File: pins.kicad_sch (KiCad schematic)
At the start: 21 parts, among them J2 Conn_01x40_Pin, J3 Conn_01x09, Q1 BC817, U11 TXS0108EPW, U8 TXS0102DCU

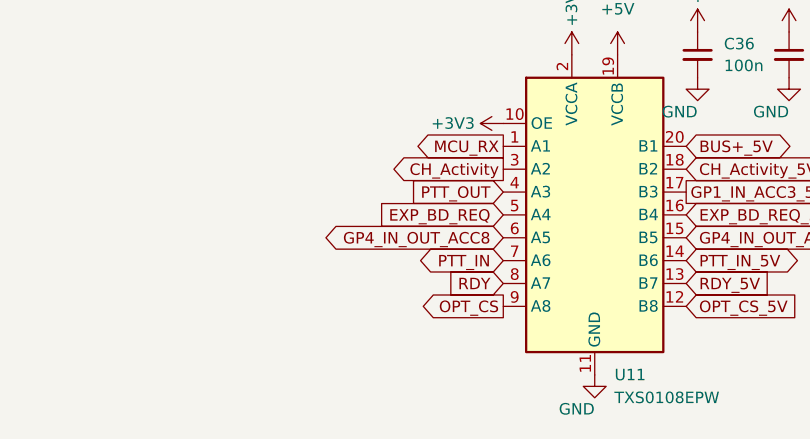
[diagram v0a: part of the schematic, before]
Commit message: end of day commit
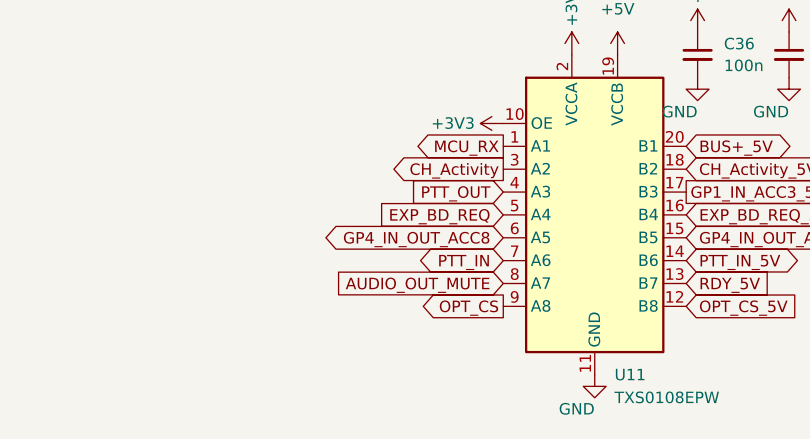
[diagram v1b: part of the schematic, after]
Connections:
- net RDY is gone; now on net AUDIO_OUT_MUTE: U11.8 (A7)
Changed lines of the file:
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@@
+		)
+	)
+	(global_label "AUDIO_OUT_MUTE"
+		(shape input)
+		(at 100.33 171.45 180)
+		(fields_autoplaced yes)
+		(effects
+			(font
+				(size 1.27 1.27)
+			)
+			(justify right)
+		)
+		(property "Intersheetrefs" "${INTERSHEET_REFS}"
+			(at 81.2581 171.45 0)
+			(effects
+				(font
+					(size 1.27 1.27)
+				)
+				(justify right)
+				(hide yes)
+			)
 		)
 	)
@@
 			(effects
 				(font
-					(size 1.27 1.27)
-				)
-				(justify right)
-				(hide yes)
-			)
-		)
-	)
-	(global_label "RDY"
-		(shape input)
-		(at 100.33 171.45 180)
-		(fields_autoplaced yes)
-		(effects
-			(font
-				(size 1.27 1.27)
-			)
-			(justify right)
-		)
-		(property "Intersheetrefs" "${INTERSHEET_REFS}"
-			(at 93.7162 171.45 0)
-			(effects
-				(font

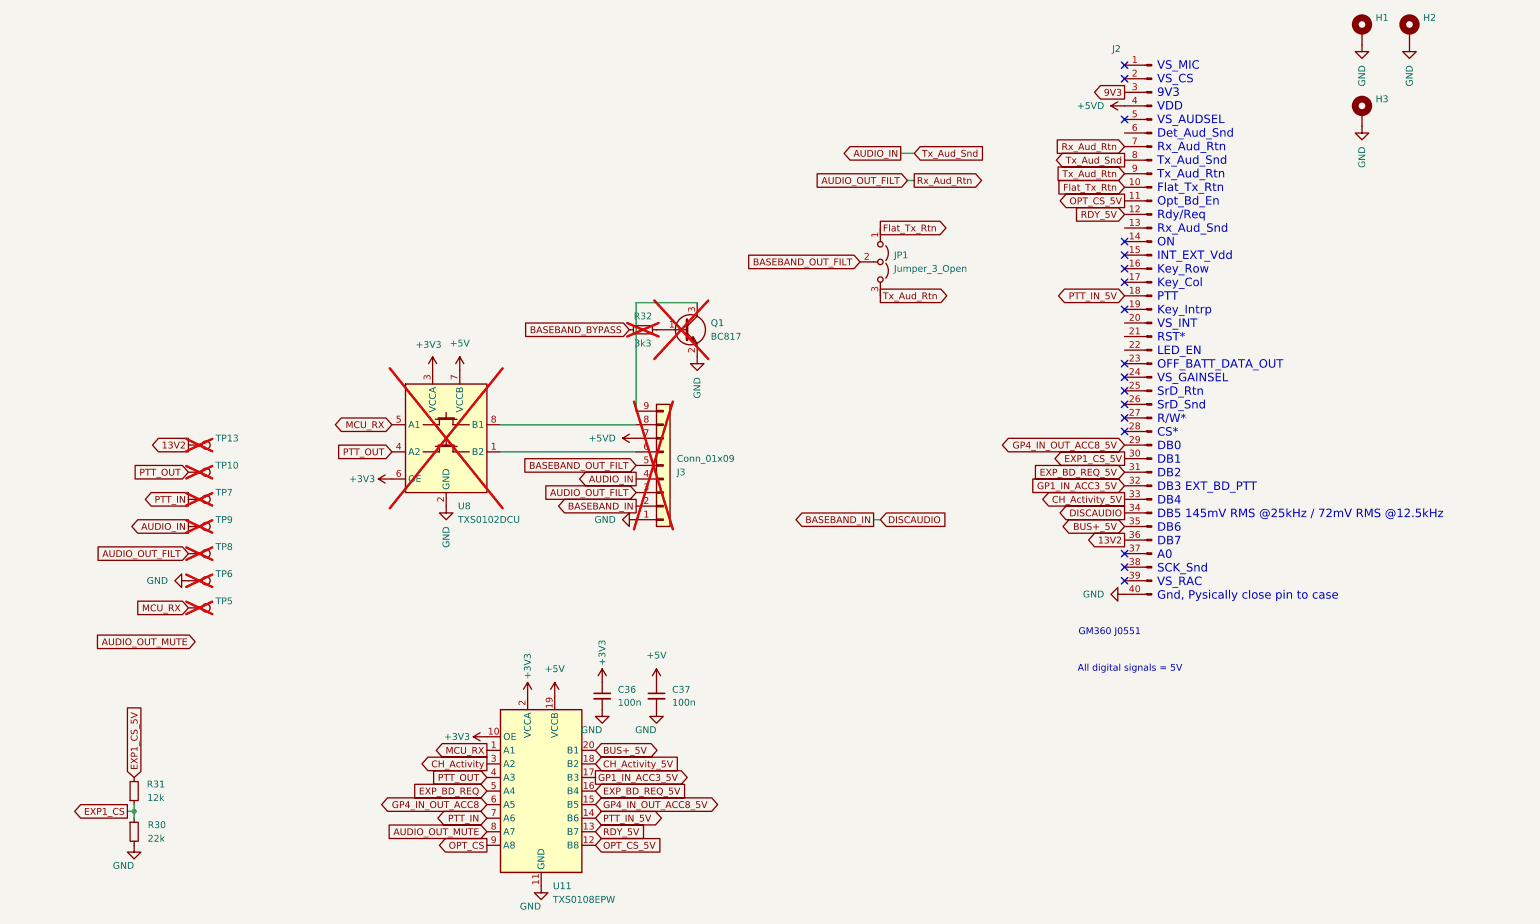
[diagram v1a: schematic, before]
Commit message: end of day commit
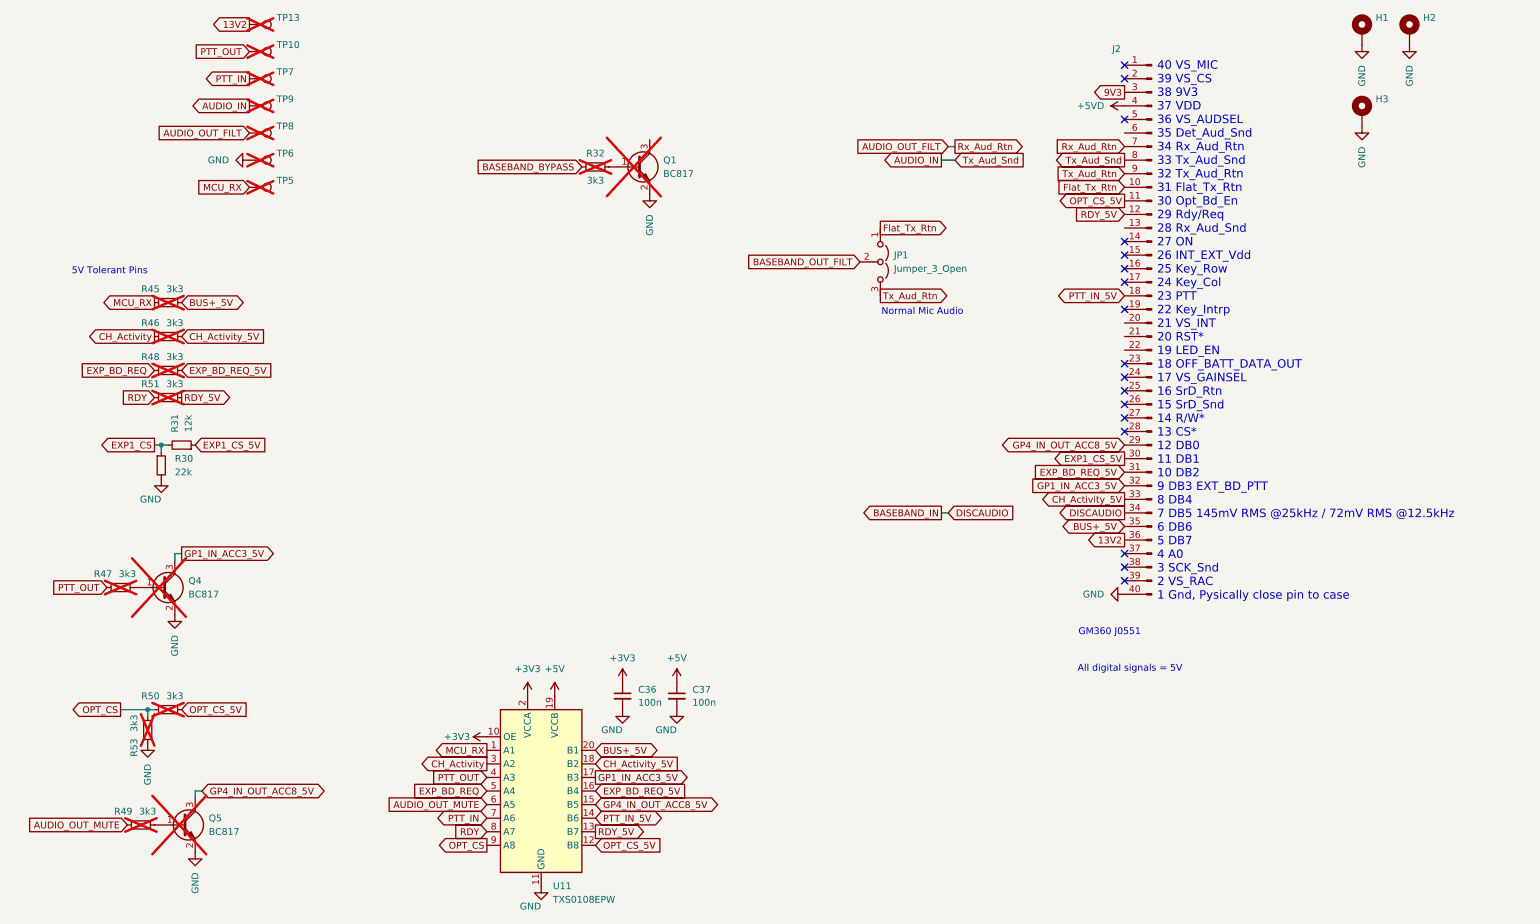
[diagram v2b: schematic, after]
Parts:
- removed J3: Conn_01x09, Connector_PinHeader_2.54mm:PinHeader_1x09_P2.54mm_Vertical, symbol Connector_Generic:Conn_01x09
- removed U8: TXS0102DCU, Package_SO:VSSOP-8_2.3x2mm_P0.5mm, symbol Logic_LevelTranslator:TXS0102DCU
- added Q4, Q5: BC817, Package_TO_SOT_SMD:SOT-23, symbol Transistor_BJT:BC817
- added R45, R46, R47, R48, R49, R50, R51, R53: 3k3, Resistor_SMD:R_0603_1608Metric_Pad0.98x0.95mm_HandSolder, symbol Device:R_Small
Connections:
- net GP4_IN_OUT_ACC8 is gone; now on net AUDIO_OUT_MUTE: U11.6 (A5)
- net AUDIO_OUT_MUTE: now also R49.1; no longer U11.8 (A7)
- net BUS+_5V: now also R45.2
- net CH_Activity: now also R46.1
- net CH_Activity_5V: now also R46.2
- net EXP1_CS: now also R31.2; no longer R31.1
- net EXP1_CS_5V: now also R31.1; no longer R31.2
- net EXP_BD_REQ: now also R48.1
- net EXP_BD_REQ_5V: now also R48.2
- net GND: now also Q4.2 (E), Q5.2 (E), R53.1
- net GP1_IN_ACC3_5V: now also Q4.3 (C)
- net GP4_IN_OUT_ACC8_5V: now also Q5.3 (C)
- net MCU_RX: now also R45.1
- net OPT_CS: now also R50.1, R53.2
- net OPT_CS_5V: now also R50.2
- net PTT_OUT: now also R47.1
- net RDY_5V: now also R51.2
- new net: Q4.1 (B), R47.2
- new net: Q5.1 (B), R49.2
- new net RDY: R51.1, U11.8 (A7)
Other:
- note added: "40 VS_MIC 39 VS_CS 38 9V3 37 VDD 36 VS_AUDSEL 35 Det_Aud_Snd 34 Rx_Aud_Rtn 33 Tx_Aud_Snd 32 Tx_Aud_Rtn 31 Flat_Tx_Rtn 30 Opt_Bd_En 29 Rdy/Req 28 Rx_Aud_Snd 27 ON 26 INT_EXT_Vdd 25 Key_Row 24 Key_Col 23 PTT 22 Key_Intrp 21 VS_INT 20 RST* 19 LED_EN 18 OFF_BATT_DATA_OUT 17 VS_GAINSEL 16 SrD_Rtn 15 SrD_Snd 14 R/W* 13 CS* 12 DB0 11 DB1 10 DB2 9 DB3 EXT_BD_PTT 8 DB4 7 DB5 145mV RMS @25kHz / 72mV RMS @1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"
- note added: "5V Tolerant Pins"
- note added: "Normal Mic Audio"
- note removed: "VS_MIC VS_CS 9V3 VDD VS_AUDSEL Det_Aud_Snd Rx_Aud_Rtn Tx_Aud_Snd Tx_Aud_Rtn Flat_Tx_Rtn Opt_Bd_En Rdy/Req Rx_Aud_Snd ON INT_EXT_Vdd Key_Row Key_Col PTT Key_Intrp VS_INT RST* LED_EN OFF_BATT_DATA_OUT VS_GAINSEL SrD_Rtn SrD_Snd R/W* CS* DB0 DB1 DB2 DB3 EXT_BD_PTT DB4 DB5 145mV RMS @25kHz / 72mV RMS @12.5kHz DB6 DB7 A0 SCK_Snd VS_RAC Gnd, Pysically close pin to case"
- moved on the sheet: C36, C37, Q1, R30, R31, R32, TP10, TP13, TP5, TP6, TP7, TP8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
